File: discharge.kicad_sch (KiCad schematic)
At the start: 5 parts, among them K1 G5LE-1

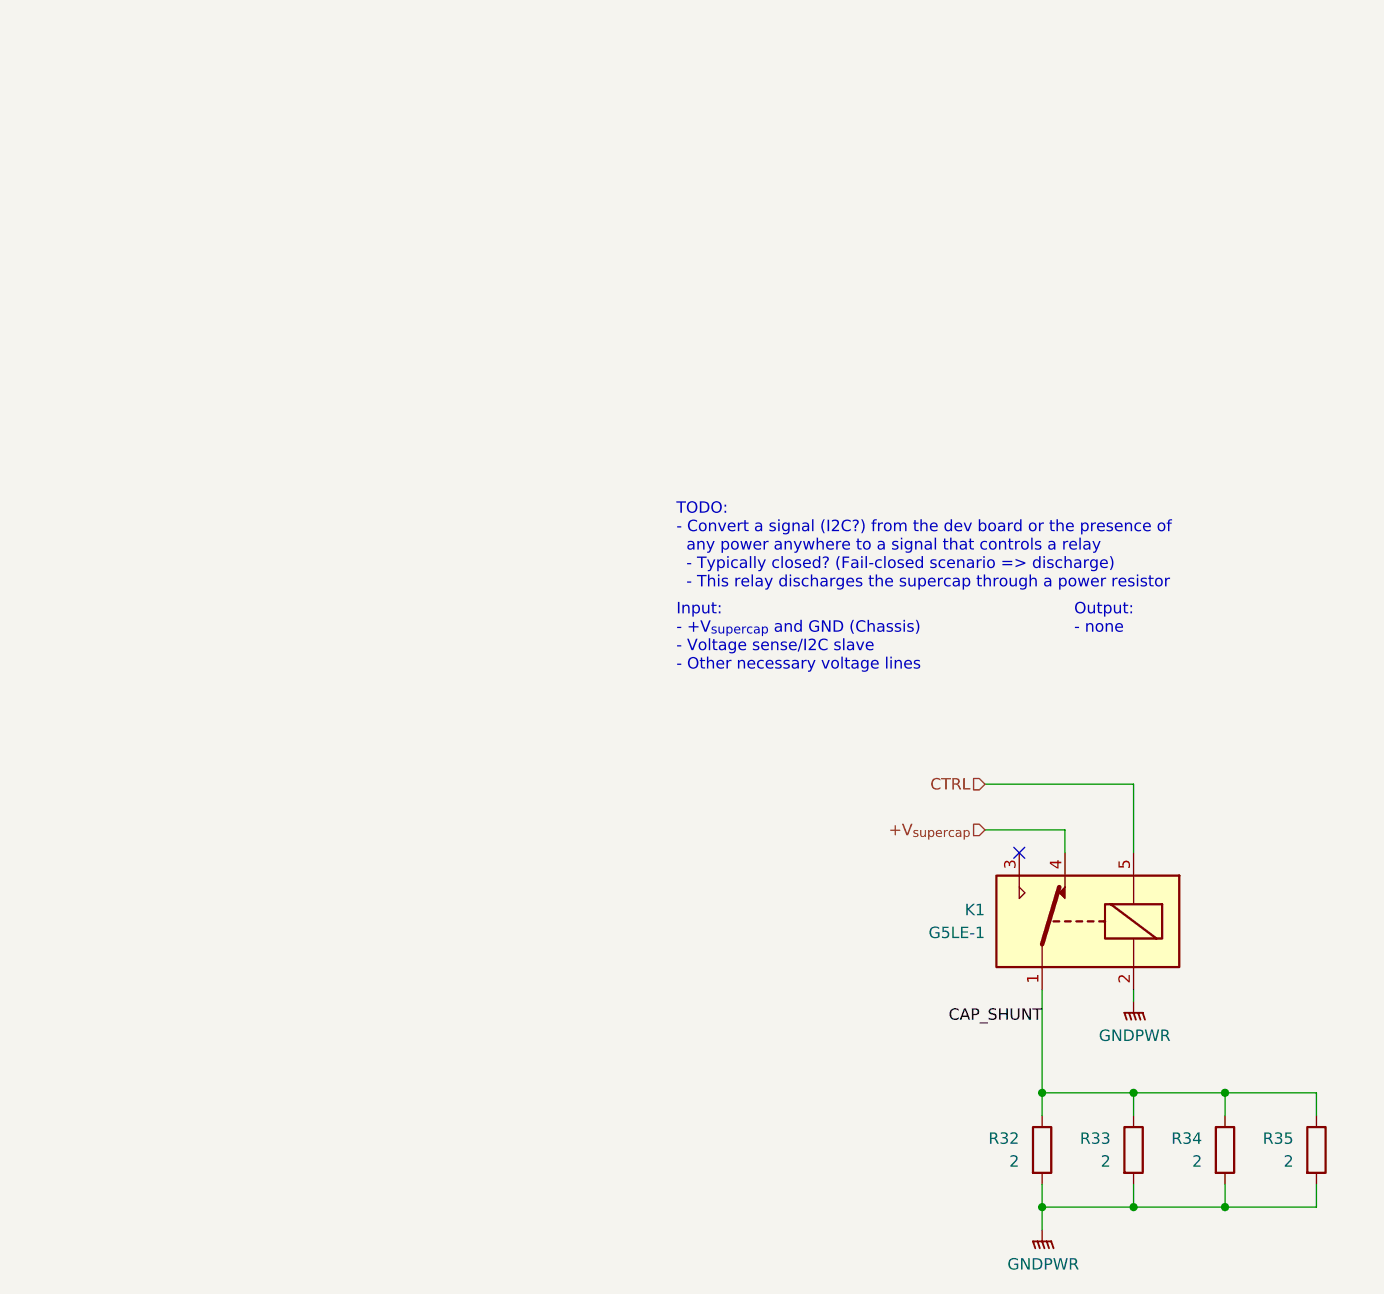
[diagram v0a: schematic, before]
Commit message: Sourcing various parts
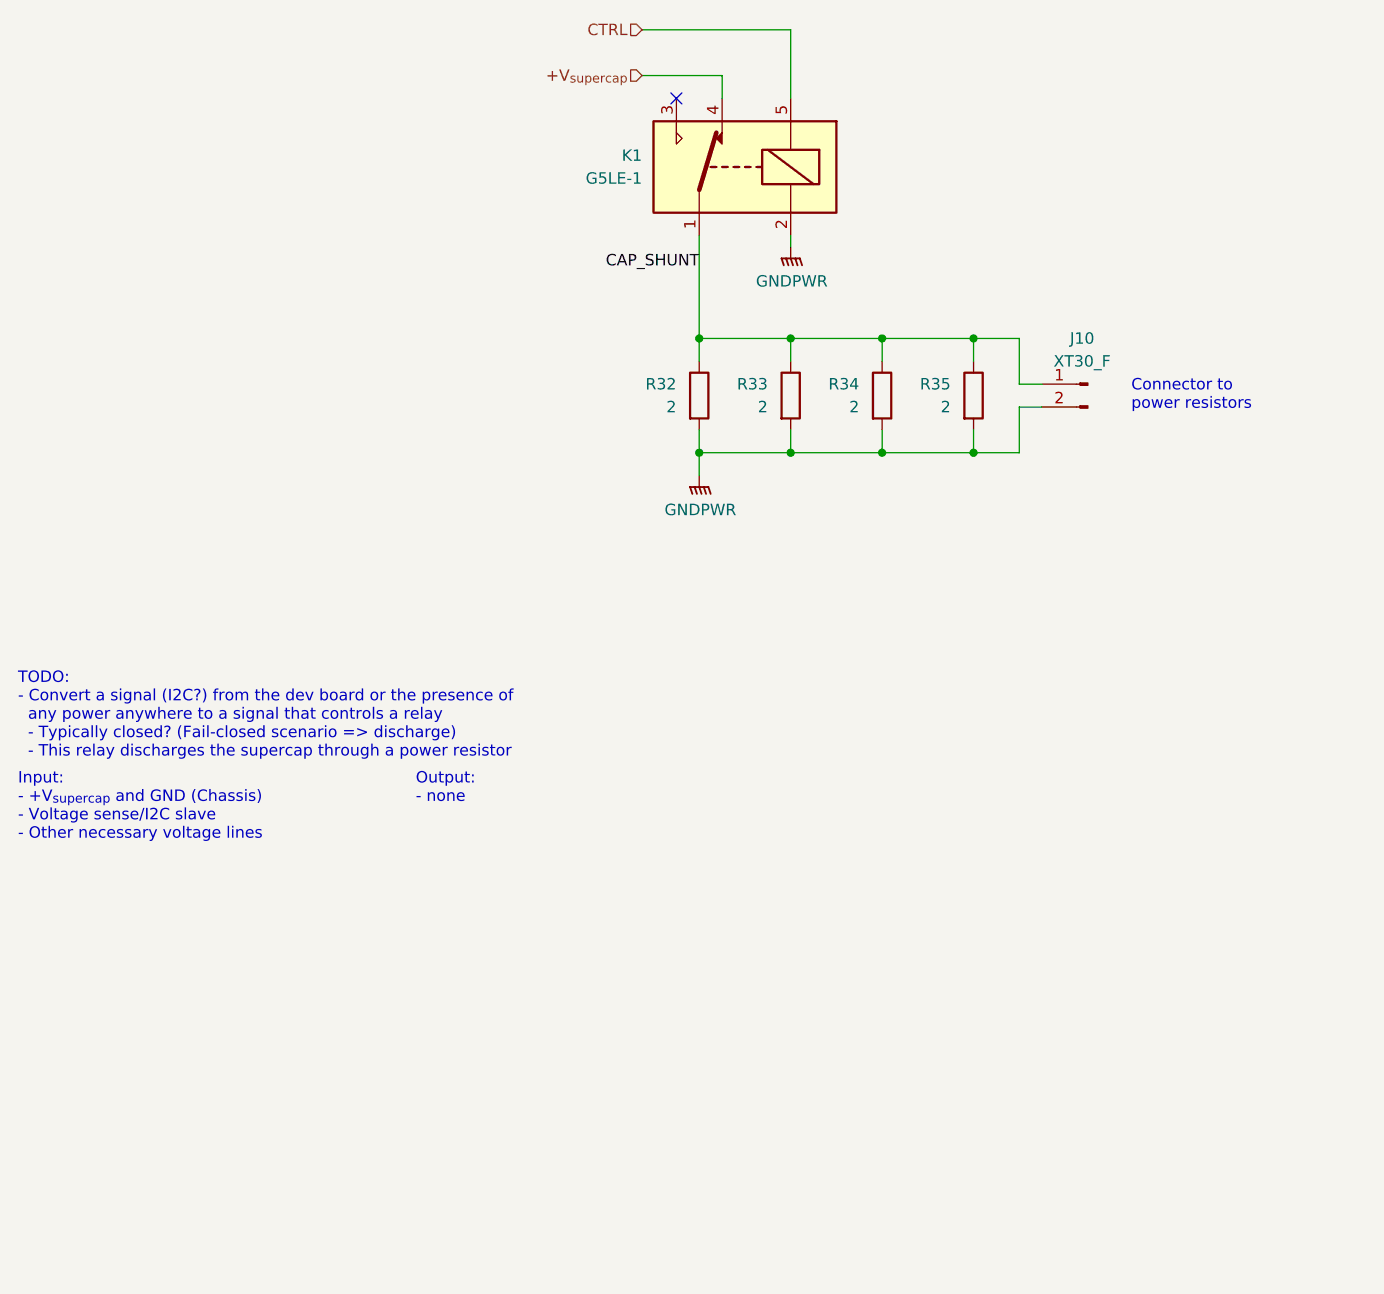
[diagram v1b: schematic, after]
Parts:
- added J10: XT30_F, Connector_AMASS:AMASS_XT30U-F_1x02_P5.0mm_Vertical, symbol Connector:Conn_01x02_Pin
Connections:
- net CAP_SHUNT: now also J10.1 (Pin_1)
- net GNDPWR: now also J10.2 (Pin_2)
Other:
- note added: "Connector to power resistors"
- moved on the sheet: K1, R32, R33, R34, R35
